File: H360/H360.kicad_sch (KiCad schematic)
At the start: 29 parts, among them J1 TYPE-C-31-M-12, J2 JST-PH 2.0, Q1 AO3401A, SW1 SW_SPST, SW2 TS-1187A-B-A-B, U1 SRV05-4-P-T7, U2 TP4056-42-ESOP8, U3 nRF52840_holyiot_18010, U4 XC6206PxxxMR

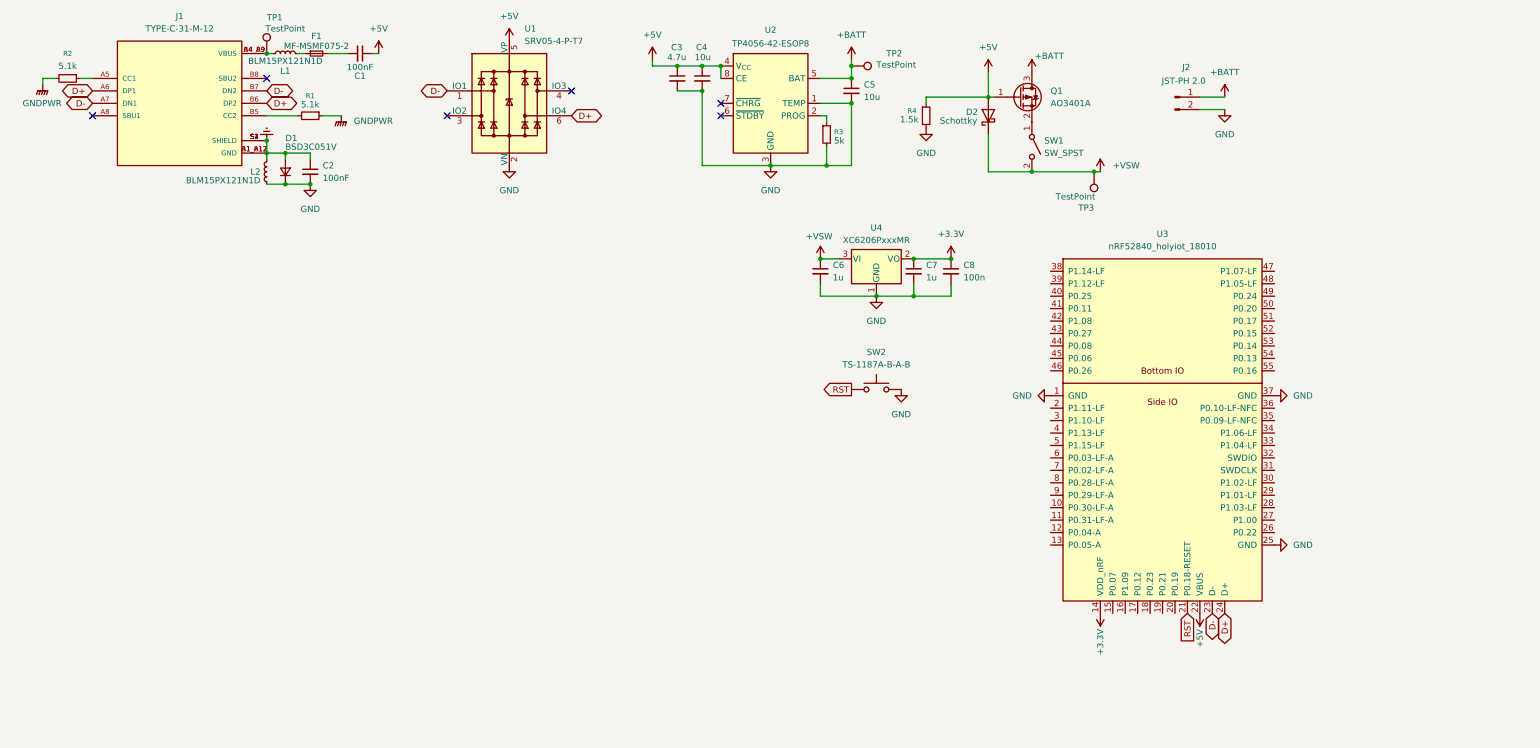
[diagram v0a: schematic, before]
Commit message: sch update
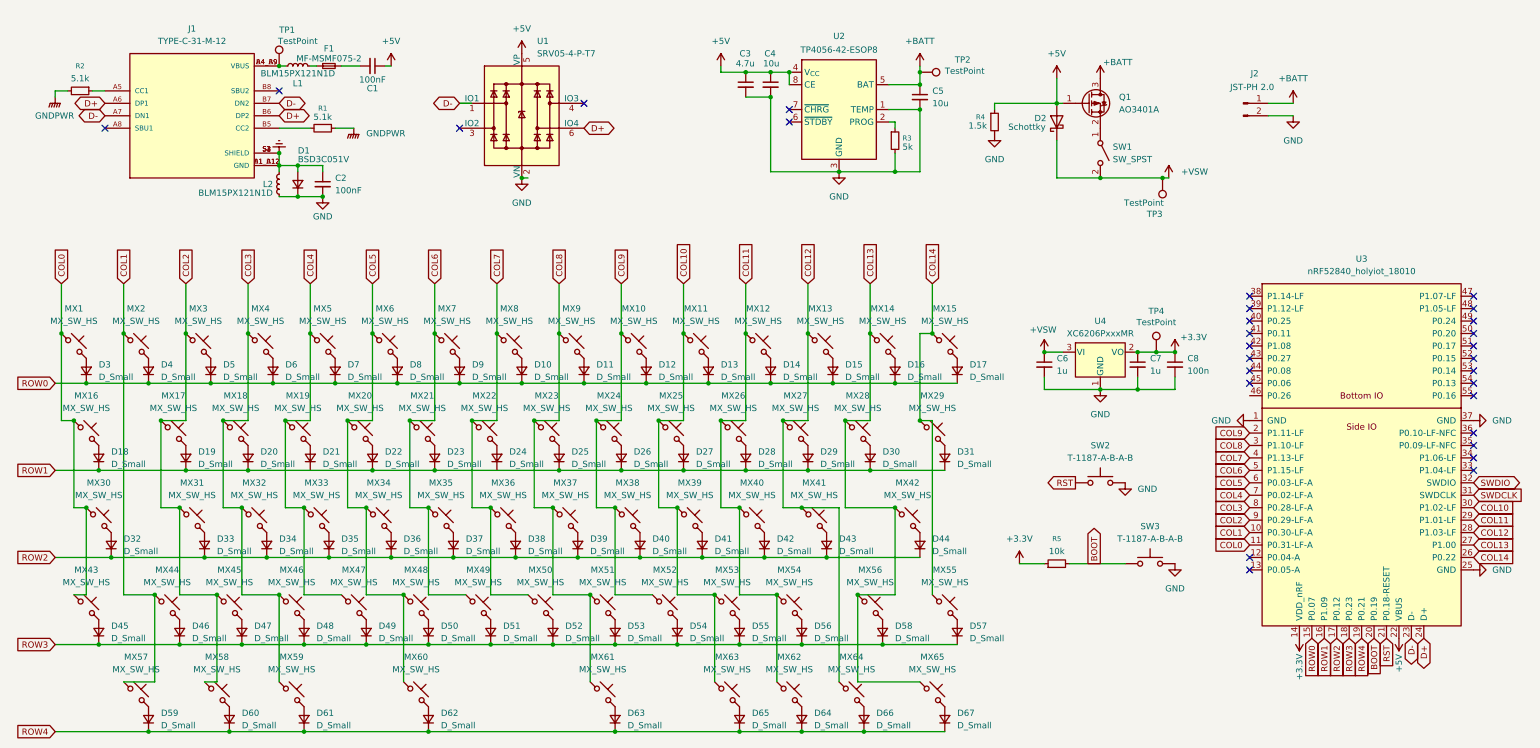
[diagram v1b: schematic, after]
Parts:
- removed SW2: TS-1187A-B-A-B, symbol Switch:SW_MEC_5G
- added D10, D11, D12, D13, D14, D15, D16, D17, D18, D19, D20, D21, D22, D23, D24, D25, D26, D27, D28, D29, D3, D30, D31, D32, D33, D34, D35, D36, D37, D38, D39, D4, D40, D41, D42, D43, D44, D45, D46, D47, D48, D49, D5, D50, D51, D52, D53, D54, D55, D56, D57, D58, D59, D6, D60, D61, D62, D63, D64, D65, D66, D67, D7, D8, D9: D_Small, symbol Device:D_Small
- added MX1, MX10, MX11, MX12, MX13, MX14, MX15, MX16, MX17, MX18, MX19, MX2, MX20, MX21, MX22, MX23, MX24, MX25, MX26, MX27, MX28, MX29, MX3, MX30, MX31, MX32, MX33, MX34, MX35, MX36, MX37, MX38, MX39, MX4, MX40, MX41, MX42, MX43, MX44, MX45, MX46, MX47, MX48, MX49, MX5, MX50, MX51, MX52, MX53, MX54, MX55, MX56, MX57, MX58, MX59, MX6, MX60, MX61, MX62, MX63, MX64, MX65, MX7, MX8, MX9: MX_SW_HS, PCM_marbastlib-mx:SW_MX_HS_CPG151101S11_1u, symbol marbastlib-mx:MX_SW_HS_CPG151101S11
- added R5: 10k, symbol Device:R_Small
- added SW2, SW3: T-1187-A-B-A-B, symbol Switch:SW_Push
- added TP4: TestPoint, symbol Connector:TestPoint
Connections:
- net +3.3V: now also R5.1, TP4.1
- net GND: now also SW2.2, SW3.2
- net RST: now also SW2.1
- net COL1: now reaches U3.10 (P0.30-LF-A)
- net COL1: now also MX2.1, MX44.1, MX57.1
- net COL0: now reaches U3.11 (P0.31-LF-A)
- net COL0: now also MX1.1, MX16.1, MX30.1, MX43.1
- net ROW0: now reaches U3.15 (P0.07)
- net ROW0: now also D10.1 (K), D11.1 (K), D12.1 (K), D13.1 (K), D14.1 (K), D15.1 (K), D16.1 (K), D17.1 (K), D3.1 (K), D4.1 (K), D5.1 (K), D6.1 (K), D7.1 (K), D8.1 (K), D9.1 (K)
- net ROW1: now reaches U3.16 (P1.09)
- net ROW1: now also D18.1 (K), D19.1 (K), D20.1 (K)
- net ROW2: now reaches U3.17 (P0.12)
- net ROW2: now also D32.1 (K), D33.1 (K), D34.1 (K), D35.1 (K), D36.1 (K), D37.1 (K), D38.1 (K), D39.1 (K), D40.1 (K), D41.1 (K), D42.1 (K), D43.1 (K), D44.1 (K)
- net ROW3: now reaches U3.18 (P0.23)
- net ROW3: now also D45.1 (K), D46.1 (K), D47.1 (K), D48.1 (K), D49.1 (K), D50.1 (K), D51.1 (K), D52.1 (K), D53.1 (K), D54.1 (K), D55.1 (K), D56.1 (K), D57.1 (K), D58.1 (K)
- net ROW4: now reaches U3.19 (P0.21)
- net ROW4: now also D59.1 (K), D60.1 (K), D61.1 (K), D62.1 (K), D63.1 (K), D64.1 (K), D65.1 (K), D66.1 (K), D67.1 (K)
- net COL9: now reaches U3.2 (P1.11-LF)
- net COL9: now also MX10.1, MX24.1, MX38.1, MX52.1
- net BOOT: now reaches U3.20 (P0.19)
- net BOOT: now also R5.2, SW3.1
- net COL14: now reaches U3.26 (P0.22)
- net COL14: now also MX15.1, MX29.1, MX55.1
- net COL13: now reaches U3.27 (P1.00)
- net COL13: now also MX14.1, MX28.1, MX42.1, MX56.1, MX65.1
- net COL12: now reaches U3.28 (P1.03-LF)
- net COL12: now also MX13.1, MX27.1, MX41.1, MX64.1
- net COL11: now reaches U3.29 (P1.01-LF)
- net COL11: now also MX12.1, MX26.1, MX40.1, MX54.1, MX62.1
- net COL8: now reaches U3.3 (P1.10-LF)
- net COL8: now also MX23.1, MX37.1, MX51.1, MX61.1, MX9.1
- net COL10: now reaches U3.30 (P1.02-LF)
- net COL10: now also MX11.1, MX25.1, MX39.1, MX53.1, MX63.1
- net SWDCLK: now reaches U3.31 (SWDCLK)
- net SWDIO: now reaches U3.32 (SWDIO)
- net COL7: now reaches U3.4 (P1.13-LF)
- net COL7: now also MX22.1, MX36.1, MX50.1, MX8.1
- net COL6: now reaches U3.5 (P1.15-LF)
- net COL6: now also MX21.1, MX35.1, MX49.1, MX7.1
- net COL5: now reaches U3.6 (P0.03-LF-A)
- net COL5: now also MX20.1, MX34.1, MX48.1, MX6.1, MX60.1
- net COL4: now reaches U3.7 (P0.02-LF-A)
- net COL4: now also MX19.1, MX33.1, MX47.1, MX5.1
- net COL3: now reaches U3.8 (P0.28-LF-A)
- net COL3: now also MX18.1, MX32.1, MX4.1, MX46.1, MX59.1
- net COL2: now reaches U3.9 (P0.29-LF-A)
- net COL2: now also MX17.1, MX3.1, MX31.1, MX45.1, MX58.1
- new net: D58.2 (A), MX56.2
- new net: D49.2 (A), MX47.2
- new net: D31.2 (A), MX29.2
- new net: D33.2 (A), MX31.2
- new net: D8.2 (A), MX6.2
- new net: D59.2 (A), MX57.2
- new net: D34.2 (A), MX32.2
- new net: D67.2 (A), MX65.2
- new net: D42.2 (A), MX40.2
- new net: D17.2 (A), MX15.2
- new net: D43.2 (A), MX41.2
- new net: D7.2 (A), MX5.2
- new net: D56.2 (A), MX54.2
- new net: D61.2 (A), MX59.2
- new net: D64.2 (A), MX62.2
- new net: D24.1 (K), D25.1 (K), D26.1 (K), D27.1 (K), D28.1 (K), D29.1 (K), D30.1 (K), D31.1 (K)
- new net: D26.2 (A), MX24.2
- new net: D65.2 (A), MX63.2
- new net: D32.2 (A), MX30.2
- new net: D66.2 (A), MX64.2
- new net: D27.2 (A), MX25.2
- new net: D60.2 (A), MX58.2
- new net: D40.2 (A), MX38.2
- new net: D63.2 (A), MX61.2
- new net: D28.2 (A), MX26.2
- new net: D4.2 (A), MX2.2
- new net: D6.2 (A), MX4.2
- new net: D19.2 (A), MX17.2
- new net: D30.2 (A), MX28.2
- new net: D9.2 (A), MX7.2
- new net: D21.1 (K), D22.1 (K), D23.1 (K)
- new net: D21.2 (A), MX19.2
- new net: D20.2 (A), MX18.2
- new net: D36.2 (A), MX34.2
- new net: D48.2 (A), MX46.2
- new net: D12.2 (A), MX10.2
- new net: D51.2 (A), MX49.2
- new net: D52.2 (A), MX50.2
- new net: D23.2 (A), MX21.2
- new net: D37.2 (A), MX35.2
- new net: D45.2 (A), MX43.2
- new net: D44.2 (A), MX42.2
- new net: D54.2 (A), MX52.2
- new net: D22.2 (A), MX20.2
- new net: D3.2 (A), MX1.2
- new net: D57.2 (A), MX55.2
- new net: D10.2 (A), MX8.2
- new net: D62.2 (A), MX60.2
- new net: D18.2 (A), MX16.2
- new net: D5.2 (A), MX3.2
- new net: D35.2 (A), MX33.2
- new net: D41.2 (A), MX39.2
- new net: D55.2 (A), MX53.2
- new net: D25.2 (A), MX23.2
- new net: D14.2 (A), MX12.2
- new net: D13.2 (A), MX11.2
- new net: D39.2 (A), MX37.2
- new net: D53.2 (A), MX51.2
- new net: D46.2 (A), MX44.2
- new net: D16.2 (A), MX14.2
- new net: D47.2 (A), MX45.2
- new net: D24.2 (A), MX22.2
- new net: D11.2 (A), MX9.2
- new net: D50.2 (A), MX48.2
- new net: D29.2 (A), MX27.2
- new net: D38.2 (A), MX36.2
- new net: D15.2 (A), MX13.2
- no-connect marks 6 -> 29
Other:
- moved on the sheet: C1, C2, C3, C4, C5, C6, C7, C8, D1, D2, F1, J1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
